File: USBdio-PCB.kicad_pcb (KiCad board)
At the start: 2 copper layers, 82.5 x 101.6 mm, 67 parts, among them IC1 ATMEGA328-P, P0 RELAY_(JSM1A-12V-4), P1 RELAY_(JSM1A-12V-4), P2 RELAY_(JSM1A-12V-4), P3 RELAY_(JSM1A-12V-4), P4 RELAY_(JSM1A-12V-4), P5 RELAY_(JSM1A-12V-4), P6 RELAY_(JSM1A-12V-4), P7 RELAY_(JSM1A-12V-4), P8 CONN_01X03, Q1 Q_NPN_BEC, Q10 Q_NPN, Q11 Q_NPN, Q12 Q_NPN, Q13 Q_NPN, Q14 Q_NPN, Q15 Q_NPN, Q16 Q_NPN, Q17 Q_NPN, Q2 Q_NPN_BEC, Q3 Q_NPN_BEC, Q4 Q_NPN_BEC, Q5 Q_NPN_BEC, Q6 Q_NPN_BEC, Q7 Q_NPN_BEC, Q8 Q_NPN_BEC, Q9 Q_NPN_BEC, U1 NCV7805BDTRKG, X1 CRYSTAL_SMD

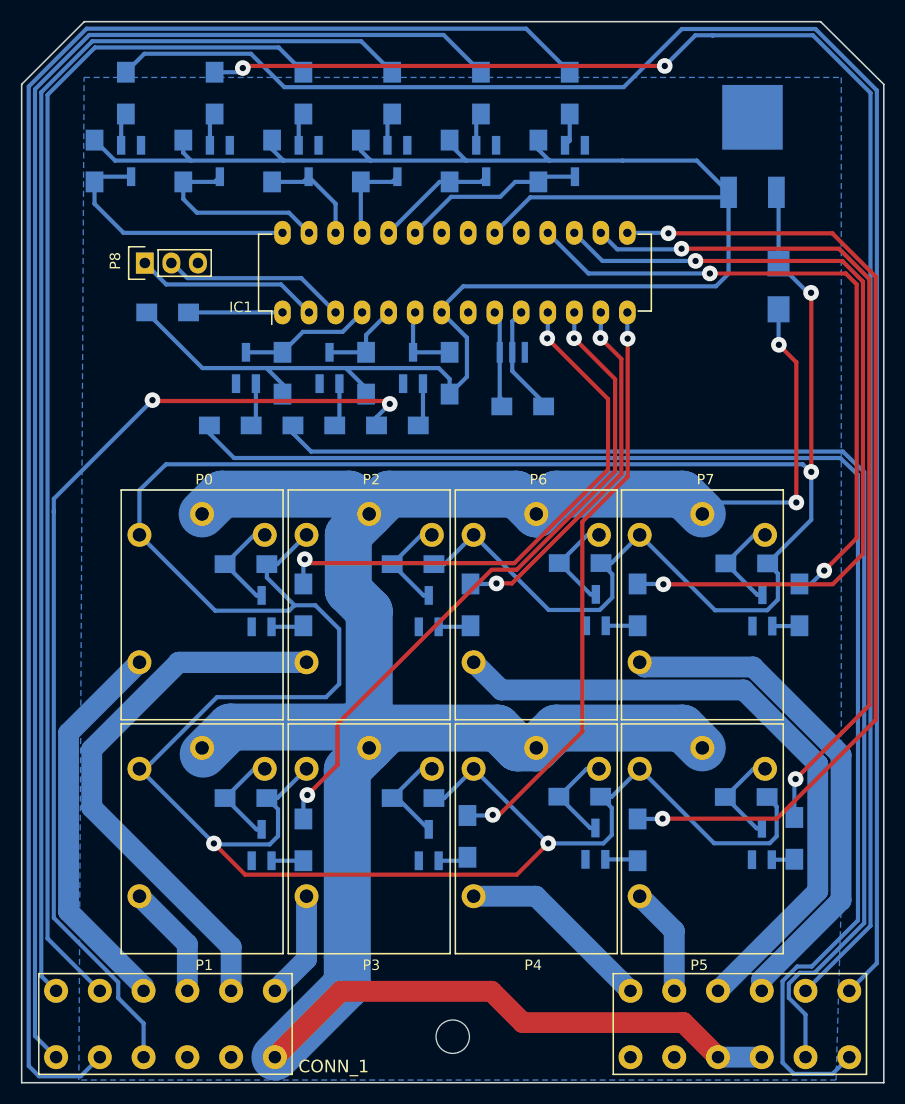
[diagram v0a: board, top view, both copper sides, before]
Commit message: finished traces
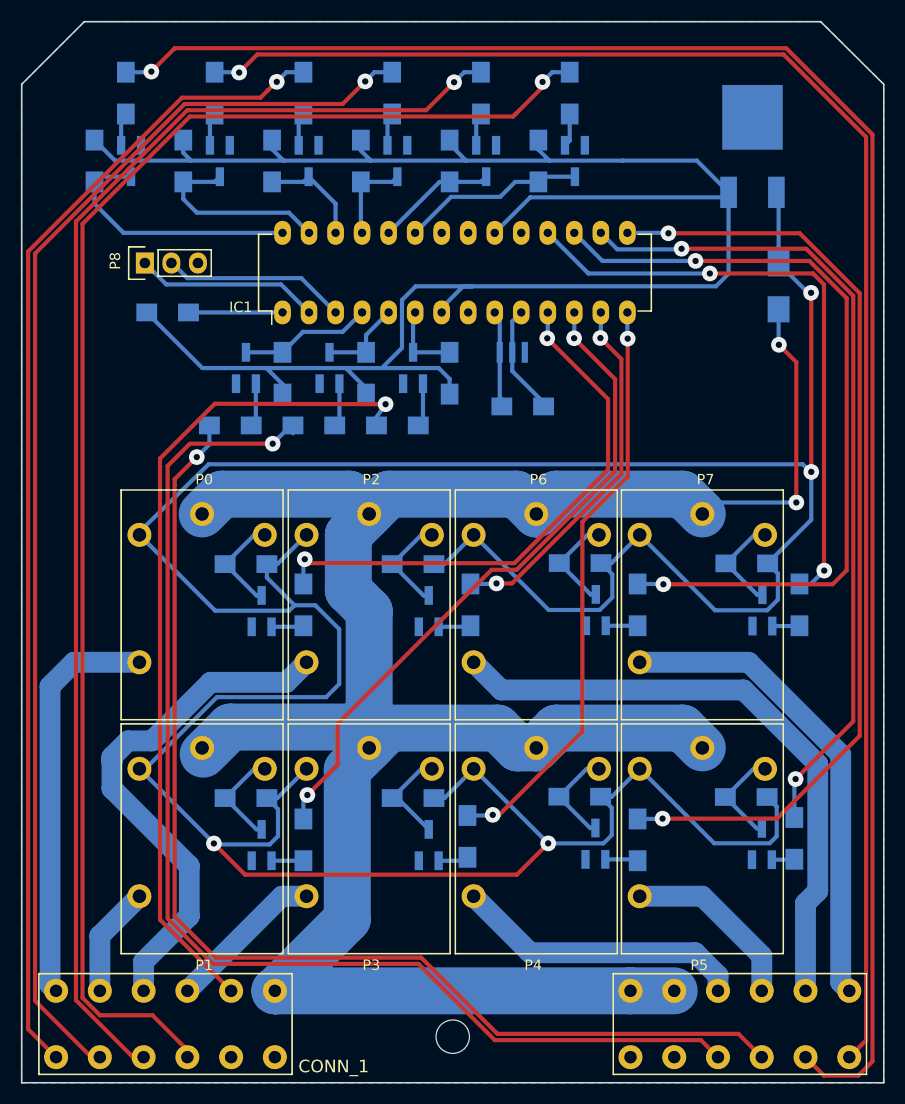
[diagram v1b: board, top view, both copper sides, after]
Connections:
- CONN_1 pad A1: Net-(CONN_1-PadA1) -> GND
- CONN_1 pad A10: RLY1 -> RLY3
- CONN_1 pad A11: RLY2 -> Net-(CONN_1-PadA11)
- CONN_1 pad A12: RLY3 -> Net-(CONN_1-PadA12)
- CONN_1 pad A2: Net-(CONN_1-PadA2) -> GND
- CONN_1 pad A3: Net-(CONN_1-PadA2) -> Net-(CONN_1-PadA3)
- CONN_1 pad A7: Net-(CONN_1-PadA7) -> RLY0
- CONN_1 pad A8: Net-(CONN_1-PadA8) -> RLY1
- CONN_1 pad A9: RLY0 -> RLY2
- CONN_1 pad B1: RLY4 -> Net-(CONN_1-PadA12)
- CONN_1 pad B10: Net-(CONN_1-PadA1) -> Net-(CONN_1-PadB10)
- CONN_1 pad B11: Net-(CONN_1-PadA2) -> GND
- CONN_1 pad B12: Net-(CONN_1-PadA2) -> GND
- CONN_1 pad B2: RLY5 -> Net-(CONN_1-PadA12)
- CONN_1 pad B3: RLY6 -> RLY4
- CONN_1 pad B4: RLY7 -> RLY5
- CONN_1 pad B5: Net-(CONN_1-PadB5) -> RLY6
- CONN_1 pad B6: Net-(CONN_1-PadB6) -> RLY7
- CONN_1 pad B9: Net-(CONN_1-PadA1) -> Net-(CONN_1-PadB9)
- D9 pad 2: Net-(CONN_1-PadA1) -> Net-(CONN_1-PadA12)
- P0 pad 1: Net-(CONN_1-PadA1) -> Net-(CONN_1-PadA12)
- P1 pad 1: Net-(CONN_1-PadA1) -> Net-(CONN_1-PadA12)
- P2 pad 1: Net-(CONN_1-PadA1) -> Net-(CONN_1-PadA12)
- P3 pad 1: Net-(CONN_1-PadA1) -> Net-(CONN_1-PadA12)
- P4 pad 1: Net-(CONN_1-PadA1) -> Net-(CONN_1-PadA12)
- P5 pad 1: Net-(CONN_1-PadA1) -> Net-(CONN_1-PadA12)
- P6 pad 1: Net-(CONN_1-PadA1) -> Net-(CONN_1-PadA12)
- P7 pad 1: Net-(CONN_1-PadA1) -> Net-(CONN_1-PadA12)
- R10 pad 2: Net-(CONN_1-PadA8) -> Net-(CONN_1-PadA6)
- R12 pad 2: Net-(CONN_1-PadB5) -> Net-(CONN_1-PadB7)
- R14 pad 2: Net-(CONN_1-PadB6) -> Net-(CONN_1-PadB8)
- R16 pad 2: Net-(CONN_1-PadB7) -> Net-(CONN_1-PadB9)
- R18 pad 2: Net-(CONN_1-PadB8) -> Net-(CONN_1-PadB10)
- R2 pad 2: Net-(CONN_1-PadA4) -> Net-(CONN_1-PadA11)
- R4 pad 2: Net-(CONN_1-PadA5) -> Net-(CONN_1-PadA3)
- R6 pad 2: Net-(CONN_1-PadA6) -> Net-(CONN_1-PadA4)
- R8 pad 2: Net-(CONN_1-PadA7) -> Net-(CONN_1-PadA5)
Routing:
- net Net-(CONN_1-PadA1): track 243.4 -> 0.00 mm, vias 2 -> 0
- net Net-(CONN_1-PadA12): track 0.00 -> 223.5 mm, vias 0 -> 2
- net Net-(CONN_1-PadB6): track 166.0 -> 0.00 mm
- net Net-(CONN_1-PadB5): track 155.2 -> 0.00 mm, vias 2 -> 0
- net Net-(CONN_1-PadA3): track 0.00 -> 139.9 mm, vias 0 -> 1
- net Net-(CONN_1-PadA7): track 123.5 -> 0.00 mm
- net Net-(CONN_1-PadB10): track 0.00 -> 115.9 mm, vias 0 -> 1
- net Net-(CONN_1-PadA8): track 115.2 -> 0.00 mm
- net Net-(CONN_1-PadB9): track 0.00 -> 111.0 mm, vias 0 -> 1
- net Net-(CONN_1-PadA11): track 0.00 -> 80.3 mm, vias 0 -> 1
- net Net-(CONN_1-PadB8): track 117.5 -> 172.3 mm, vias 0 -> 1
- net Net-(CONN_1-PadA5): track 157.6 -> 121.4 mm, vias 0 -> 1
- net Net-(CONN_1-PadA4): track 96.0 -> 128.0 mm, vias 2 -> 1
- net Net-(CONN_1-PadA6): track 139.8 -> 111.8 mm, vias 0 -> 1
- net Net-(CONN_1-PadB7): track 132.1 -> 155.2 mm, vias 0 -> 1
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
